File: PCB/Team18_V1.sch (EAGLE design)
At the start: 1 part, among them IC1 STM32F746ZGT6

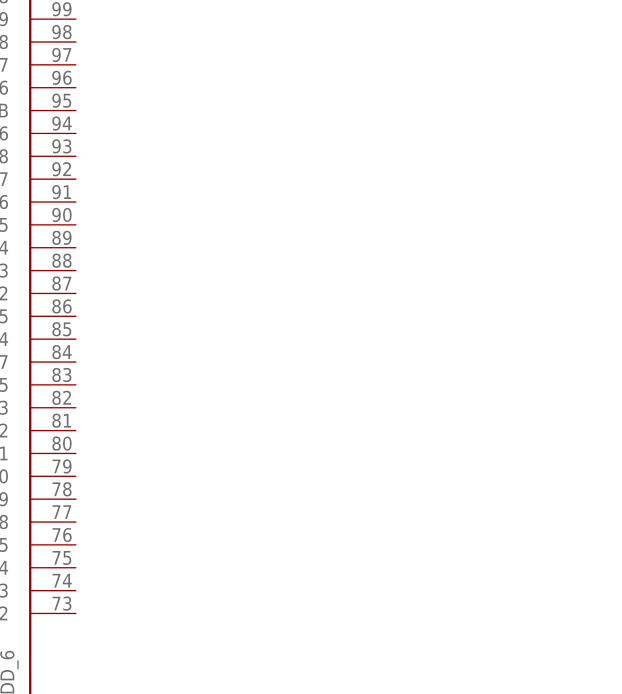
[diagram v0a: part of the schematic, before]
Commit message: pcbFiles
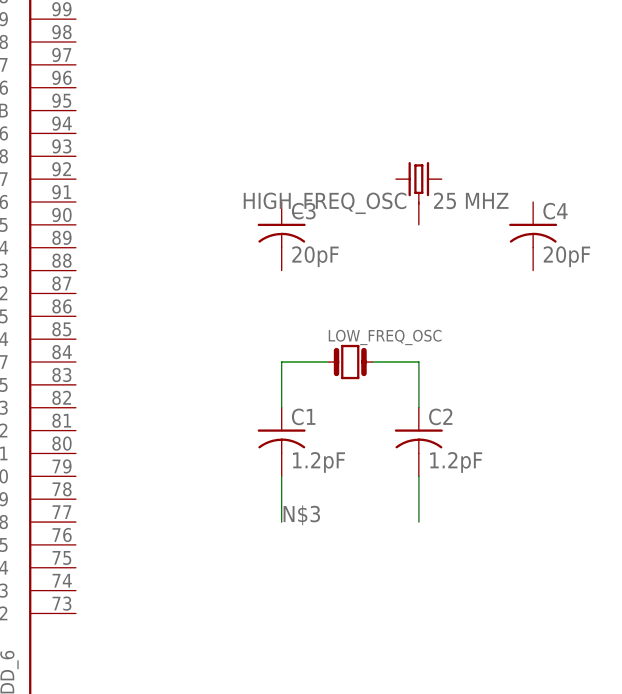
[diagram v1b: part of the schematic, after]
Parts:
- added C1, C2: 1.2pF, adafruit:C-USC0805
- added C3, C4: 20pF, adafruit:C-USC0805
- added HIGH_FREQ_OSC: 25 MHZ, SparkFun-Clocks:CRYSTAL-26MHZSMD-3.2X2.5
- added LOW_FREQ_OSC: (no value), mbed-HDK-Oscillator:GENERIC-CRYSTAL_FC135
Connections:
- new net N$1: C1.1, LOW_FREQ_OSC.1
- new net N$2: C2.1, LOW_FREQ_OSC.2
- new net N$3: C1.2
- new net N$4: C2.2

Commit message: PCB
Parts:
- added C10, C11, C12, C13, C14, C15, C5, C6, C7, C8: 100nF, rcl:C-EUC0805
- added C16, C17: 2.2uF, audio amplifier example:CAP_CERAMIC0805-NOOUTLINE
- added C9: (no value), rcl:C-EUC0805
- added FERRITE_BEAD: (no value), Wurth_Elektronik_Passive_rev18f:WE-CBA_0805_782853112_HC
- added P1: 1-1473005-4, Rpi-DDR2:1-1473005-4
- added R1: 0, audio amplifier example:R-US_R0805
- added R2: 1k, audio amplifier example:R-US_R0805
- added R3: 10k, audio amplifier example:R-US_R0805
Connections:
- removed net N$3: C1.2
- removed net N$4: C2.2
- new net 3.3V: P1.191, P1.192, P1.193, P1.194, R3.2
- new net GND: C1.2, C10.2, C11.2, C12.2, C13.2, C14.1, C15.1, C16.2, C17.2, C2.2, C3.2, C4.2, C5.1, C6.1, C7.1, C8.2, C9.2, HIGH_FREQ_OSC.3, IC1.VSSA, IC1.VSS_1, IC1.VSS_2, IC1.VSS_3, IC1.VSS_4, IC1.VSS_5, IC1.VSS_7, IC1.VSS_8, IC1.VSS_9, P1.1, P1.103, P1.104, P1.109, P1.110, P1.115, P1.116, P1.121, P1.122, P1.127, P1.13, P1.133, P1.134, P1.139, P1.14, P1.140, P1.145, P1.146, P1.151, P1.152, P1.157, P1.163, P1.164, P1.169, P1.170, P1.181, P1.182, P1.187, P1.188, P1.19, P1.195, P1.196, P1.20, P1.25, P1.26, P1.31, P1.32, P1.37, P1.38, P1.43, P1.44, P1.49, P1.50, P1.55, P1.56, P1.61, P1.62, P1.67, P1.68, P1.7, P1.73, P1.74, P1.79, P1.8, P1.80, P1.85, P1.86, P1.91, P1.92, P1.97, P1.98, R2.2
- new net OSC32_IN: C1.1, IC1.PC14, LOW_FREQ_OSC.1
- new net OSC32_OUT: C2.1, IC1.PC15, LOW_FREQ_OSC.2
- new net OSC_IN: C3.1, HIGH_FREQ_OSC.1, IC1.PHO
- new net OSC_OUT: C4.1, HIGH_FREQ_OSC.2, IC1.PH1
- new net RUN: P1.177, R3.1
- new net USB_OTGID: P1.168, R2.1
- new net VBAT: P1.197, P1.198, P1.199, P1.200
- new net VBATSTM: IC1.PE6
- new net VDD: C10.1, C11.1, C12.1, C13.1, C14.2, C15.2, C5.2, C6.2, C7.2, C8.1, C9.1, FERRITE_BEAD.1, IC1.VDD_1, IC1.VDD_10, IC1.VDD_11, IC1.VDD_2, IC1.VDD_3, IC1.VDD_4, IC1.VDD_5, IC1.VDD_6, IC1.VDD_7, IC1.VDD_8, IC1.VDD_9
- new net VDDA: FERRITE_BEAD.2, IC1.VDDA, R1.1
- new net VREF: IC1.VREF+, R1.2
- net N$1: now also C16.1, IC1.VCAP_1; no longer C1.1, LOW_FREQ_OSC.1
- net N$2: now also C17.1, IC1.VCAP_2; no longer C2.1, LOW_FREQ_OSC.2
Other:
- moved on the sheet: C1, C2, C3, C4, HIGH_FREQ_OSC, LOW_FREQ_OSC
